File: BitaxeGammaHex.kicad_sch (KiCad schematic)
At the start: 9 parts, among them J5 Conn_02x03_Counter_Clockwise

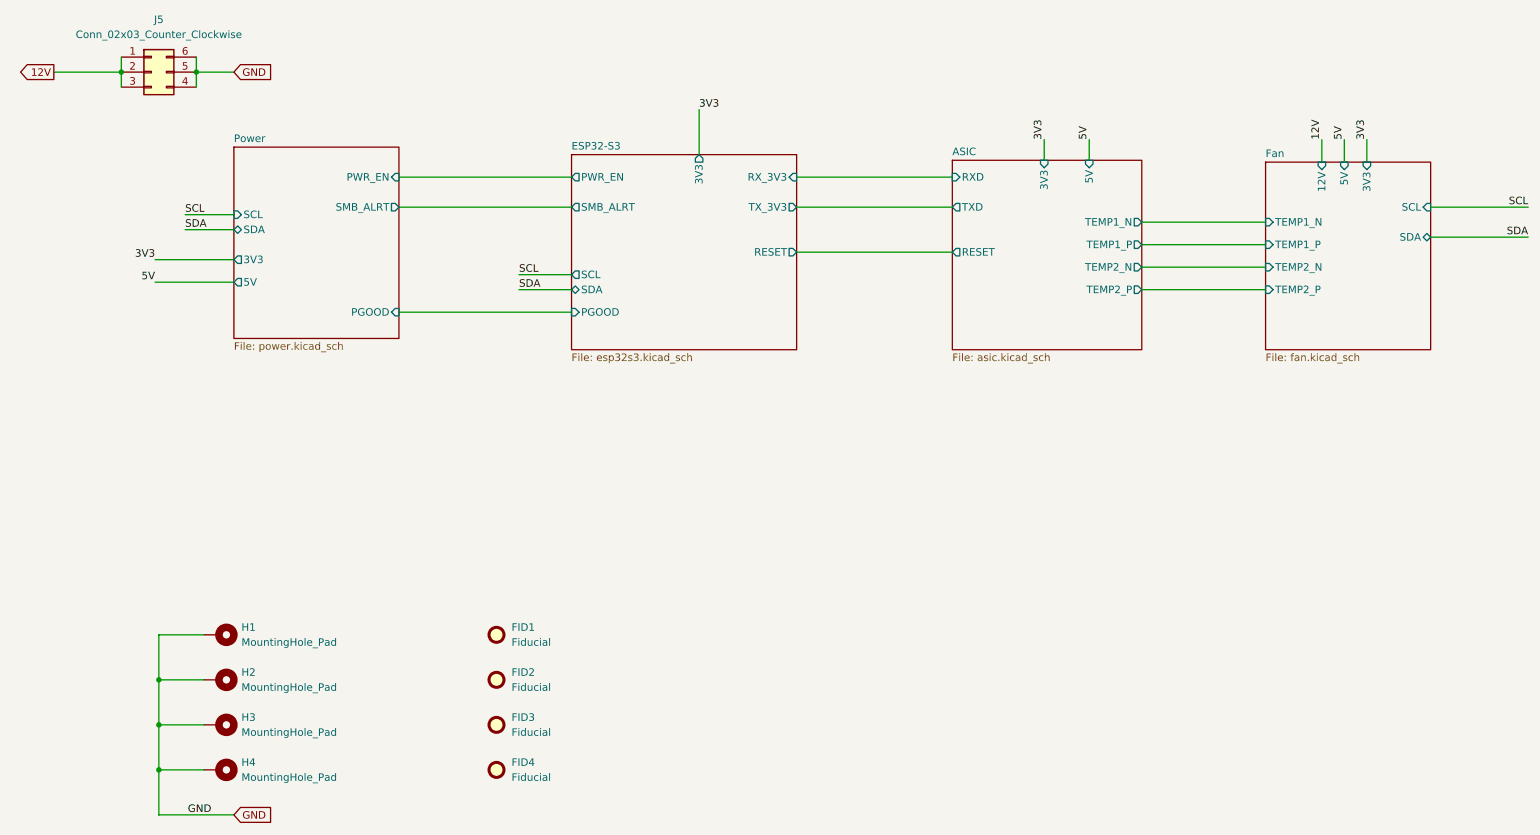
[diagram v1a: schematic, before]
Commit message: power sheet schematic cleanup
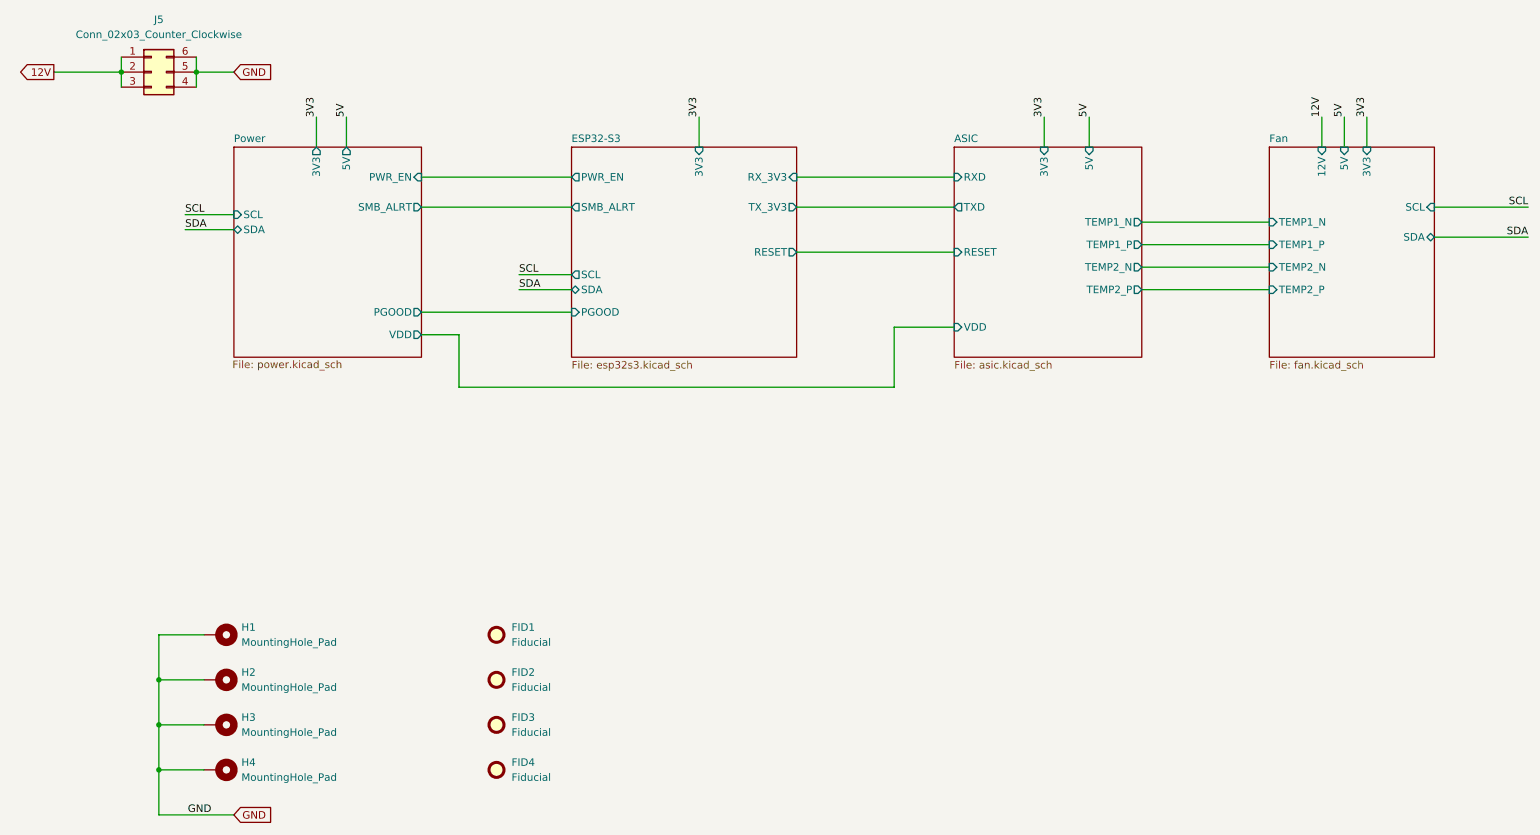
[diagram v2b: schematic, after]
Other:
- sheet ASIC ports: added VDD; removed none
- sheet Power ports: added VDD; removed none
